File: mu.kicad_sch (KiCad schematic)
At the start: 70 parts, among them J1 JTAG-10 PIN, J2 XT30PW-M, J3 U.FL-R-SMT-1_10_, J4 ESQ-110-X-X-D, J5 ESQ-110-X-X-D, U1 STM32F042F6P6, U10 TLV3603QDCKRQ1, U11 SN74LVC1G74DCUT, U13 MCP4921-E/SN, U14 BMP390, U2 MAX5026EUT_T, U3 MICROFC-60035-SMT-TR1, U4 TLV70433DBVT, U5 W25Q128JVS, U6 OPA656NB/250, U8 LT3045xDD, U9 sn65hvd230

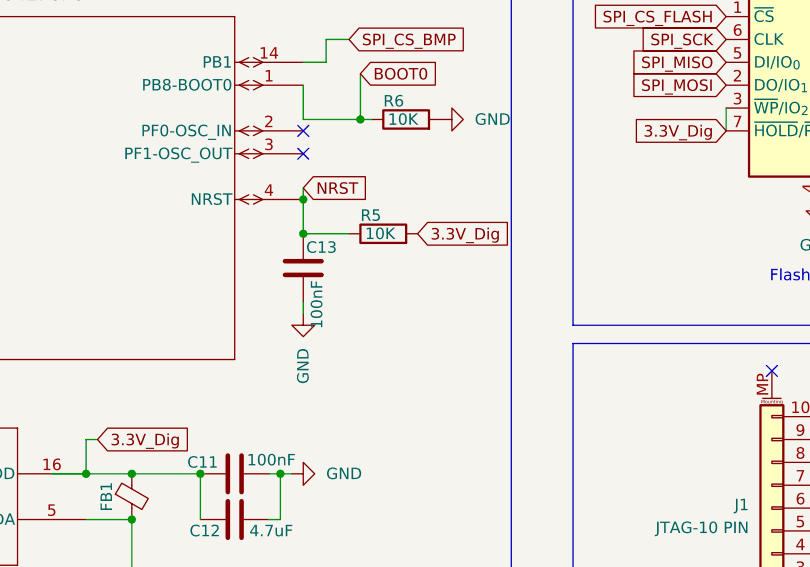
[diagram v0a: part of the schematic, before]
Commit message: fixed the connector
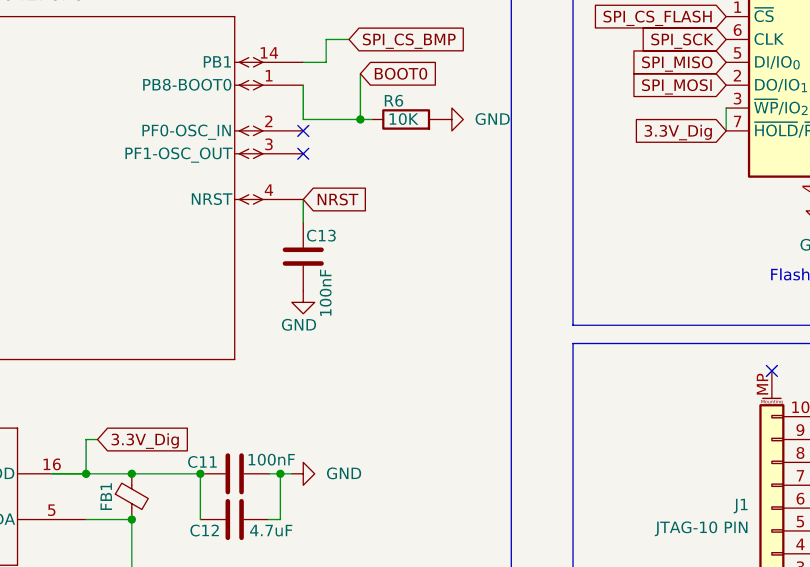
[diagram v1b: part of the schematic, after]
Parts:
- removed R5: 10K, Resistor_SMD:R_0402_1005Metric, symbol Device:R
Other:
- moved on the sheet: C13
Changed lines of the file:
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@@
 	)
 	(junction
-		(at 113.03 190.5)
-		(diameter 0)
-		(color 0 0 0 0)
-	)
-	(junction
 		(at 33.02 132.08)
 		(diameter 0)
@@
 	)
 	(junction
-		(at 113.03 194.31)
-		(diameter 0)
-		(color 0 0 0 0)
-	)
-	(junction
 		(at 99.06 62.23)
 		(diameter 0)
@@
 	(wire
 		(pts
-			(xy 113.03 201.93) (xy 113.03 203.2)
-		)
-		(stroke
-			(width 0)
-			(type default)
-		)
-	)
-	(wire
-		(pts
 			(xy 194.31 128.27) (xy 194.31 129.54)
 		)
@@
 	(wire
 		(pts
-			(xy 119.38 181.61) (xy 120.65 181.61)
+			(xy 113.03 190.5) (xy 113.03 193.04)
 		)
 		(stroke
@@
 	(wire
 		(pts
-			(xy 113.03 194.31) (xy 118.11 194.31)
+			(xy 119.38 181.61) (xy 120.65 181.61)
 		)
 		(stroke
@@
 	(wire
 		(pts
-			(xy 113.03 189.23) (xy 113.03 190.5)
-		)
-		(stroke
-			(width 0)
-			(type default)
-		)
-	)
-	(wire
-		(pts
 			(xy 72.39 119.38) (xy 81.28 119.38)
 		)
@@
 	(wire
 		(pts
-			(xy 113.03 190.5) (xy 113.03 194.31)
-		)
-		(stroke
-			(width 0)
-			(type default)
-		)
-	)
-	(wire
-		(pts
 			(xy 231.14 176.53) (xy 234.95 176.53)
 		)
@@
 	(global_label "NRST"
 		(shape input)
-		(at 113.03 189.23 0)
+		(at 113.03 190.5 0)
 		(fields_autoplaced yes)
 		(effects
@@
 		)
 		(property "Intersheetrefs" "${INTERSHEET_REFS}"
-			(at 120.7928 189.23 0)
+			(at 120.7928 190.5 0)
 			(effects
 				(font
@@
 		)
 	)
-	(global_label "3.3V_Dig"
-		(shape input)
-		(at 125.73 194.31 0)
-		(fields_autoplaced yes)
-		(effects
-			(font
-				(size 1.27 1.27)
-			)
-			(justify left)
-		)
-		(property "Intersheetrefs" "${INTERSHEET_REFS}"
-			(at 136.819 194.31 0)
-			(effects
-				(font
-					(size 1.27 1.27)
-				)
-				(justify left)
-				(hide yes)
-			)
-		)
-	)
 	(global_label "HV"
 		(shape input)
@@
 	(symbol
 		(lib_id "Device:C")
-		(at 113.03 198.12 0)
+		(at 113.03 196.85 0)
 		(unit 1)
 		(exclude_from_sim no)
@@
 		(dnp no)
 		(property "Reference" "C13"
-			(at 115.062 195.834 0)
+			(at 115.062 194.564 0)
 			(effects
 				(font
@@
 		)
 		(property "Value" "100nF"
-			(at 114.554 202.184 90)
+			(at 115.57 200.914 90)
 			(effects
 				(font
@@
 		)
 		(property "Footprint" "Capacitor_SMD:C_0402_1005Metric"
-			(at 113.9952 201.93 0)
+			(at 113.9952 200.66 0)
 			(effects
 				(font
@@
 		)
 		(property "Datasheet" "~"
-			(at 113.03 198.12 0)
+			(at 113.03 196.85 0)
 			(effects
 				(font
@@
 		)
 		(property "Description" "Unpolarized capacitor"
-			(at 113.03 198.12 0)
+			(at 113.03 196.85 0)
 			(effects
 				(font
@@
 	(symbol
 		(lib_id "power:GND")
-		(at 113.03 203.2 0)
+		(at 113.03 200.66 0)
 		(unit 1)
 		(exclude_from_sim no)
@@
 		(on_board yes)
 		(dnp no)
-		(fields_autoplaced yes)
 		(property "Reference" "#PWR013"
-			(at 113.03 209.55 0)
+			(at 113.03 207.01 0)
 			(effects
 				(font
@@
 		)
 		(property "Value" "GND"
-			(at 113.0301 207.01 90)
+			(at 114.554 204.47 0)
 			(effects
 				(font
@@
 		)
 		(property "Footprint" ""
-			(at 113.03 203.2 0)
+			(at 113.03 200.66 0)
 			(effects
 				(font
@@
 		)
 		(property "Datasheet" ""
-			(at 113.03 203.2 0)
+			(at 113.03 200.66 0)
 			(effects
 				(font
@@
 		)
 		(property "Description" "Power symbol creates a global label with name \"GND\" , ground"
-			(at 113.03 203.2 0)
+			(at 113.03 200.66 0)
 			(effects
 				(font
@@
 					(unit 1)
 				)
-			)
-		)
-	)
-	(symbol
-		(lib_id "Device:R")
-		(at 121.92 194.31 90)
-		(unit 1)
-		(exclude_from_sim no)
-		(in_bom yes)
-		(on_board yes)
-		(dnp no)
-		(property "Reference" "R5"
-			(at 119.38 192.278 90)
-			(effects
-				(font
-					(size 1.27 1.27)
-				)
-				(justify right)
-			)
-		)
-		(property "Value" "10K"
-			(at 119.888 194.31 90)
-			(effects
-				(font
-					(size 1.27 1.27)
-				)
-				(justify right)
-			)
-		)
-		(property "Footprint" "Resistor_SMD:R_0402_1005Metric"
-			(at 121.92 196.088 90)
-			(effects
-				(font
-					(size 1.27 1.27)
-				)
-				(hide yes)
-			)
-		)
-		(property "Datasheet" "~"
-			(at 121.92 194.31 0)
-			(effects
-				(font
-					(size 1.27 1.27)
-				)
-				(hide yes)
-			)
-		)
-		(property "Description" "Resistor"
-			(at 121.92 194.31 0)
-			(effects
-				(font
-					(size 1.27 1.27)
-				)
-				(hide yes)
-			)
-		)
-		(pin "1"
-		)
-		(pin "2"
-		)
-		(instances
-			(project "mu"
-				(path "/0020f91a-50ae-478d-8303-55d8991d2d34"
-					(reference "R5")
-					(unit 1)
-				)
